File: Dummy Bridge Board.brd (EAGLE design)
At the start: 86.4 x 113.7 mm, 102 parts, among them J2 5787834-1, U14 ADUM3160BRWZ-RL, U21 CD4050BD, U22 PDS1-S5-S5-M-TR, U28 FT4232HL, U29 SN74HC595DR, U30 LP5907MFX-3.3/NOPB, U49 TL7712A-SOIC, U9 TPS54540DDARQ1, Y2 CX3225GB12000P0HPQCC

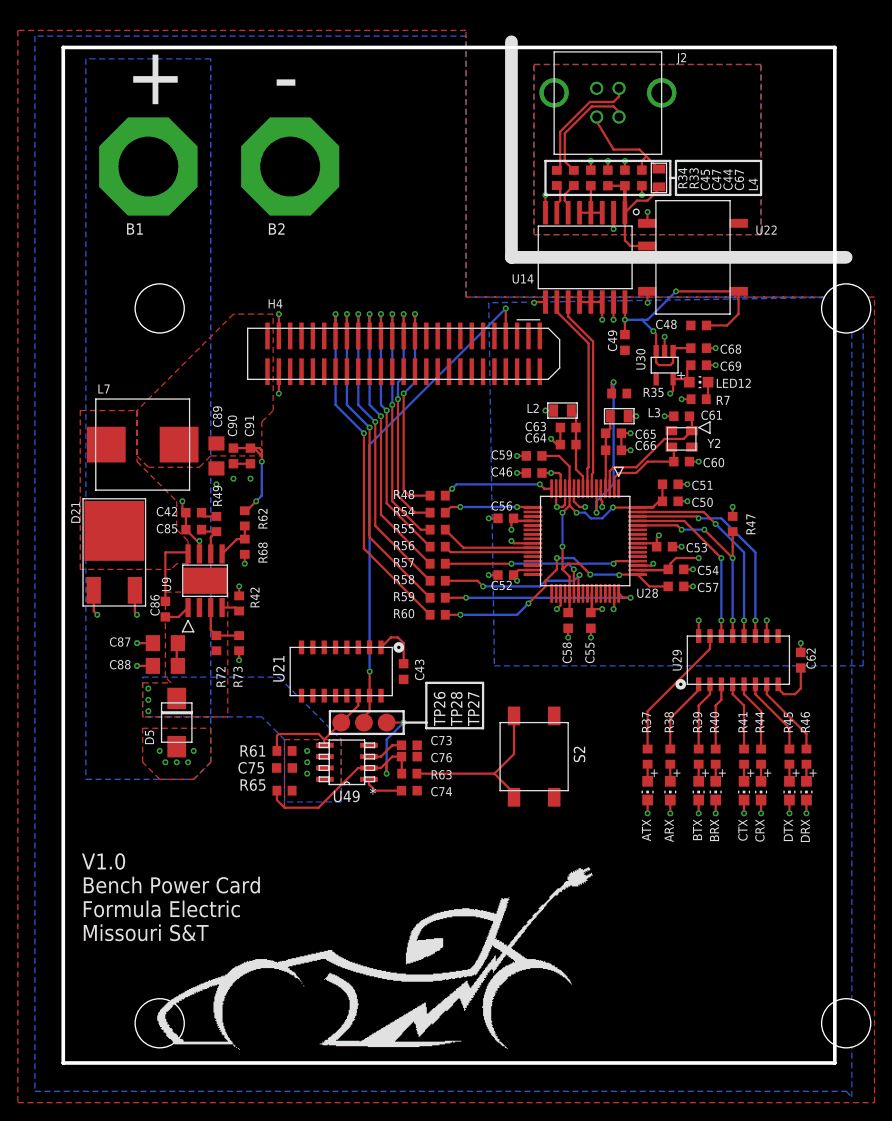
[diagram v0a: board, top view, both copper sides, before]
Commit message: BOM Exported and minor board change- ready to order
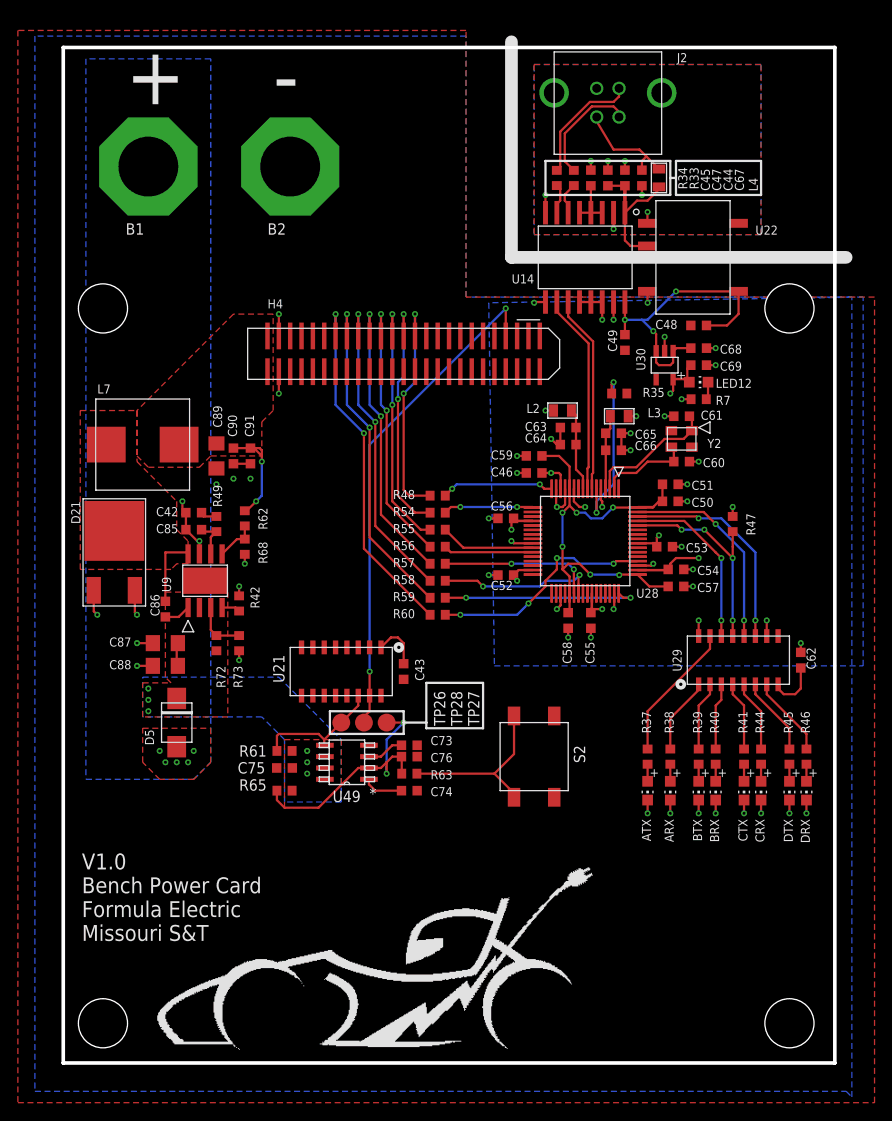
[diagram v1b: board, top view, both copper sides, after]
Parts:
- moved H2 6.35 mm to (47.6, 41.3)
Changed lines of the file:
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@@
 <attribute name="PARTNO" value="CX3225GB12000P0HPQCC" x="69.215" y="69.85" size="1.778" layer="27" rot="R180" display="off"/>
 </element>
-<element name="H2" library="FormE" package="CARCONTROLLER-REF" value="CARCONTROLLER-REF" x="53.975" y="41.275" smashed="yes"/>
+<element name="H2" library="FormE" package="CARCONTROLLER-REF" value="CARCONTROLLER-REF" x="47.625" y="41.275" smashed="yes"/>
 <element name="D5" library="FormE" package="SOD-128" value="PMEG3030EP,115" x="12.7" y="38.1" rot="R90">
 <attribute name="PARTNO" value="PMEG3030EP,115" x="12.7" y="31.115" size="1.016" layer="27" rot="R90" display="off"/>
